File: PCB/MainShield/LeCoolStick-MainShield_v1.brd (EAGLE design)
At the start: 50.8 x 50.8 mm, 16 parts

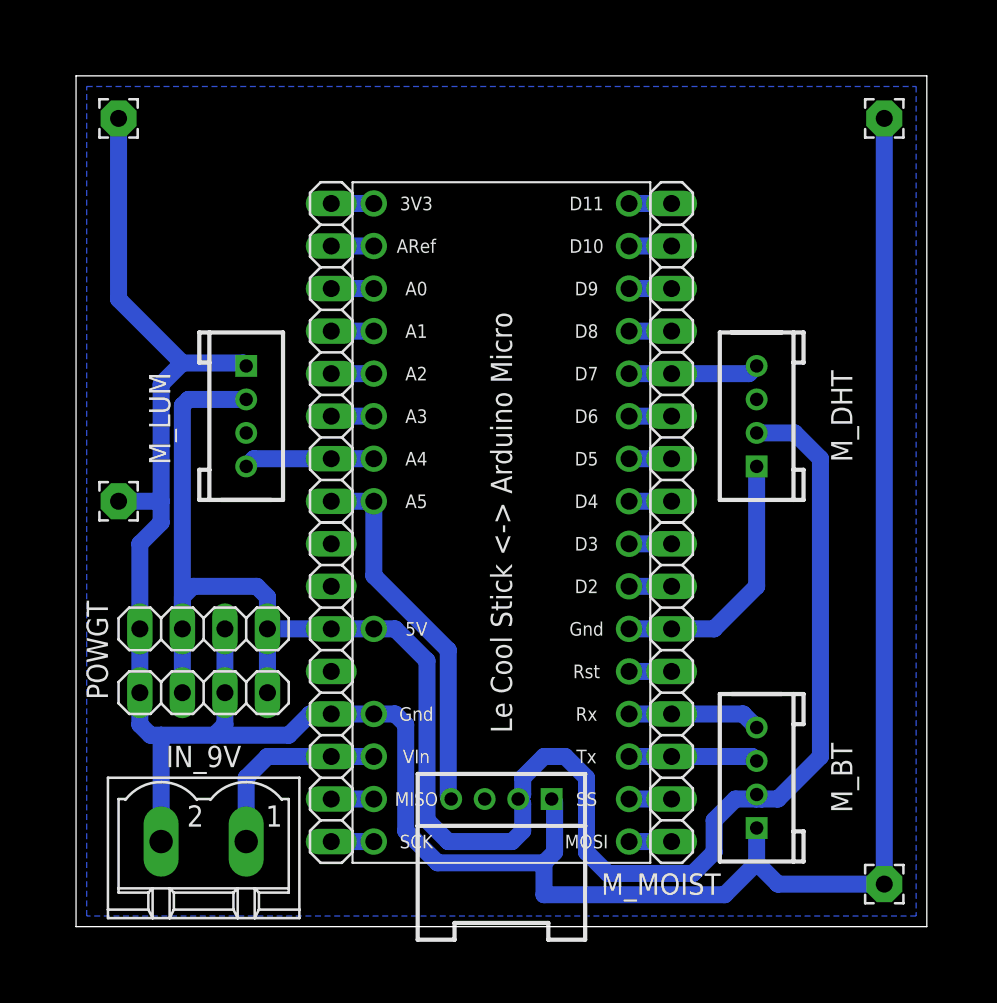
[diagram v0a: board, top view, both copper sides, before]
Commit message: Le Cool Stick - PCB V1.1
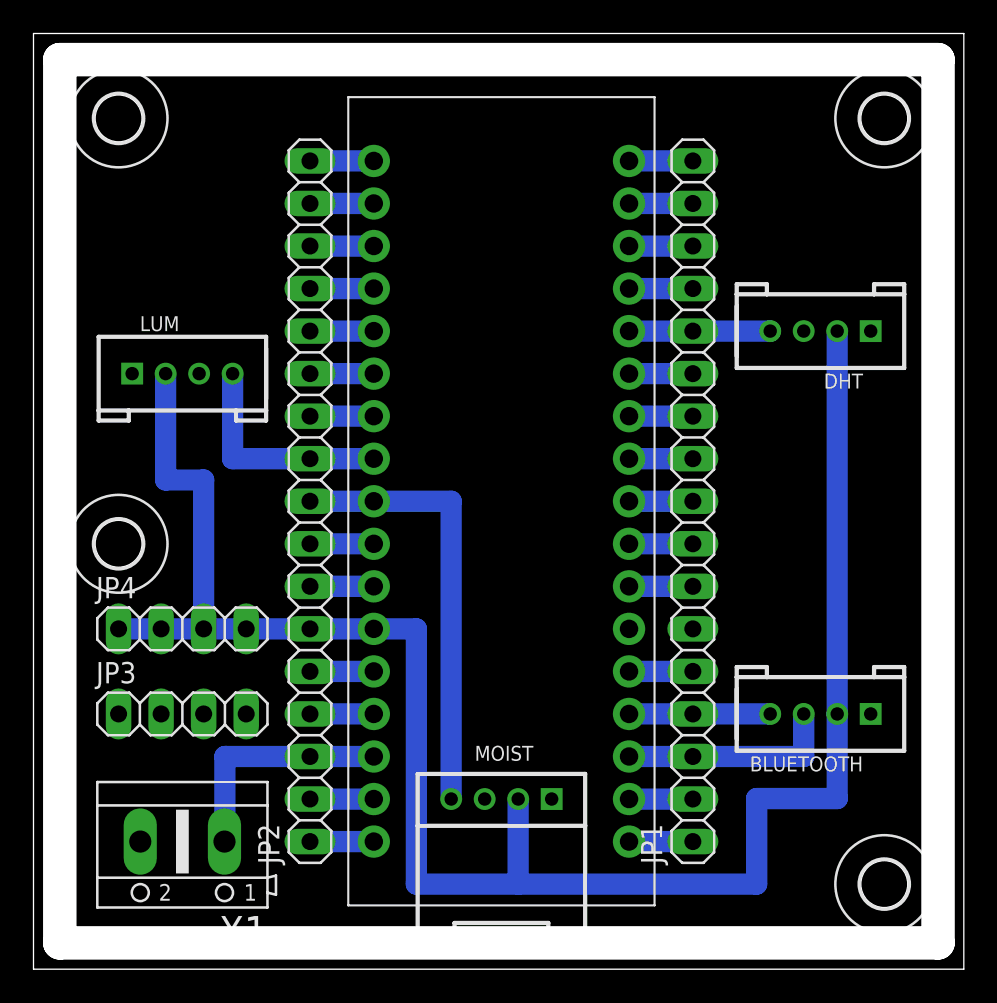
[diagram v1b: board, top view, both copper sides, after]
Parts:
- removed IN_9V: MSTBV2, LaCoolCo_Library:MSTBV2
- removed M_ANG, M_DIG, M_POWBT, M_POWSD: (no value), LaCoolCo_Library:1X08
- removed M_BT, M_DHT, M_LUM: (no value), LaCoolCo_Library:4P-2.0
- removed M_MOIST: (no value), LaCoolCo_Library:4P-2.0-90D
- removed PAD1, PAD2, PAD3, PAD4: WIREPAD2,15/1,0, LaCoolCo_Library:WIREPAD-2,15/1,0
- removed PCB1: SHIELD_MICRO, LaCoolCo_Library:SHIELD_MICRO
- removed POWGT, POWGT_1: (no value), LaCoolCo_Library:1X04
- added BLUETOOTH, DHT, LUM: 4P-2.0, Seeed-OPL-Connector:HW4-2.0
- added H1, H2, H3, H4: MOUNT-HOLE2.8, holes:2,8
- added JP1, JP2: (no value), pinhead:1X17
- added JP3, JP4: (no value), pinhead:1X04
- added MOIST: 4P-2.0-90D, Seeed-OPL-Connector:HW4-2.0-90D
- added U$1: ARDUINOMICRO, adafruit:ARDUINOMICRO
- added X1: (no value), con-ptr500:AK500/2
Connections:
- removed net +V1: M_BT.2, M_DHT.2, M_LUM.2, M_MOIST.2, M_POWSD.3, PCB1.+5V, POWGT.2, POWGT.4, POWGT_1.2, POWGT_1.4
- removed net A0: M_ANG.3, PCB1.A0
- removed net A1: M_ANG.4, PCB1.A1
- removed net A2: M_ANG.5, PCB1.A2
- removed net A3: M_ANG.6, PCB1.A3
- removed net A4: M_ANG.7, M_LUM.4, PCB1.A4
- removed net A5: M_ANG.8, M_MOIST.4, PCB1.A5
- removed net ARD_3V3: M_ANG.1, PCB1.3V3
- removed net AREF: M_ANG.2, PCB1.REF
- removed net D10: M_DIG.2, PCB1.D10
- removed net D11: M_DIG.1, PCB1.D11
- removed net D2: M_POWBT.2, PCB1.D2
- removed net D3: M_POWBT.1, PCB1.D3
- removed net D4: M_DIG.8, PCB1.D4
- removed net D5: M_DIG.7, PCB1.D5
- removed net D6: M_DIG.6, PCB1.D6
- removed net D7: M_DHT.4, M_DIG.5, PCB1.D7
- removed net D8: M_DIG.4, PCB1.D8
- removed net D9: M_DIG.3, PCB1.D9
- removed net GND_V1: IN_9V.2, M_BT.1, M_DHT.1, M_LUM.1, M_MOIST.1, M_POWBT.3, M_POWSD.5, PAD1.1, PAD2.1, PAD3.1, PAD4.1, PCB1.GND, PCB1.GND., POWGT.1, POWGT.3, POWGT_1.1, POWGT_1.3
- removed net MISO: M_POWSD.7, PCB1.MISO]
- removed net MOSI: M_POWBT.8, PCB1.MOSI
- removed net RST: M_POWBT.4, PCB1.RST
- removed net RX1: M_BT.4, M_POWBT.5, PCB1.RX1
- removed net SCK: M_POWSD.8, PCB1.SCK
- removed net SS: M_POWBT.7, PCB1.SS
- removed net TX1: M_BT.3, M_POWBT.6, PCB1.TX1
- removed net VIN: IN_9V.1, M_POWSD.6, PCB1.VIN
- new net +5V: BLUETOOTH.2, DHT.2, JP2.6, JP4.1, JP4.2, JP4.3, JP4.4, LUM.2, MOIST.2, U$1.P$23
- new net GND: BLUETOOTH.1, DHT.1, JP1.6, JP2.4, JP3.1, JP3.2, JP3.3, JP3.4, LUM.1, MOIST.1, U$1.P$12, U$1.P$21, X1.2
- new net N$1: JP2.9, MOIST.4, U$1.P$26
- new net N$10: JP1.7, U$1.P$11
- new net N$11: JP1.8, U$1.P$10
- new net N$12: JP1.9, U$1.P$9
- new net N$13: JP1.10, U$1.P$8
- new net N$14: JP1.11, U$1.P$7
- new net N$15: JP1.12, U$1.P$6
- new net N$16: JP1.14, U$1.P$4
- new net N$17: JP1.15, U$1.P$3
- new net N$18: JP1.16, U$1.P$2
- new net N$19: JP1.17, U$1.P$1
- new net N$2: JP2.10, LUM.4, U$1.P$27
- new net N$20: JP2.1, U$1.P$18
- new net N$21: JP2.2, U$1.P$19
- new net N$22: JP2.5, U$1.P$13
- new net N$24: JP2.7, U$1.P$24
- new net N$25: JP2.8, U$1.P$25
- new net N$26: JP2.11, U$1.P$28
- new net N$27: JP2.12, U$1.P$29
- new net N$28: JP2.13, U$1.P$30
- new net N$29: JP2.14, U$1.P$31
- new net N$3: DHT.4, JP1.13, U$1.P$5
- new net N$30: JP2.15, U$1.P$32
- new net N$31: JP2.16, U$1.P$33
- new net N$32: JP2.17, U$1.P$34
- new net N$4: BLUETOOTH.4, JP1.4, U$1.P$14
- new net N$5: BLUETOOTH.3, JP1.3, U$1.P$15
- new net N$6: JP1.1, U$1.P$17
- new net N$7: JP1.2, U$1.P$16
- new net N$8: JP1.5, U$1.P$22
- new net VCC: JP2.3, U$1.P$20, X1.1
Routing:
- net GND_V1: track 181.8 -> 0.00 mm
- net +V1: track 114.5 -> 0.00 mm
- net +5V: track 0.00 -> 113.7 mm
- net N$1: track 0.00 -> 26.2 mm
- net A5: track 22.2 -> 0.00 mm
- net VCC: track 0.00 -> 14.0 mm
- net N$2: track 0.00 -> 13.5 mm
- net N$5: track 0.00 -> 13.0 mm
- net VIN: track 12.0 -> 0.00 mm
- net N$3: track 0.00 -> 8.44 mm
- net N$4: track 0.00 -> 8.43 mm
- net RX1: track 7.96 -> 0.00 mm
- net A4: track 7.81 -> 0.00 mm
- net D7: track 7.81 -> 0.00 mm
- net TX1: track 7.73 -> 0.00 mm
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- added copper zone on layer 16, net GND
- removed copper zone on layer 16, net GND_V1
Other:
- board size 50.8 x 50.8 mm -> 55.5 x 55.9 mm
